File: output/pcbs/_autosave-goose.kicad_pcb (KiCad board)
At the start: 2 copper layers, 135.7 x 97.7 mm, 39 parts

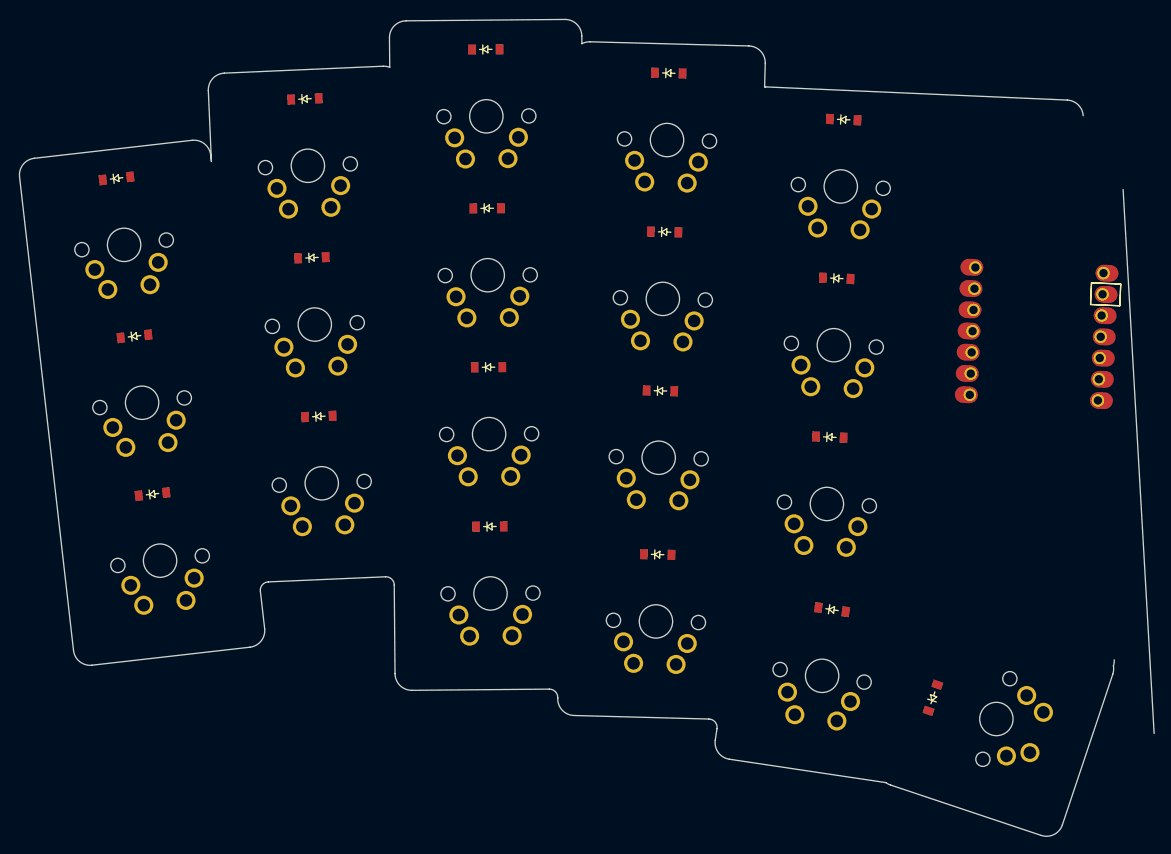
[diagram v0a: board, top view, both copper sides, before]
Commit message: partial
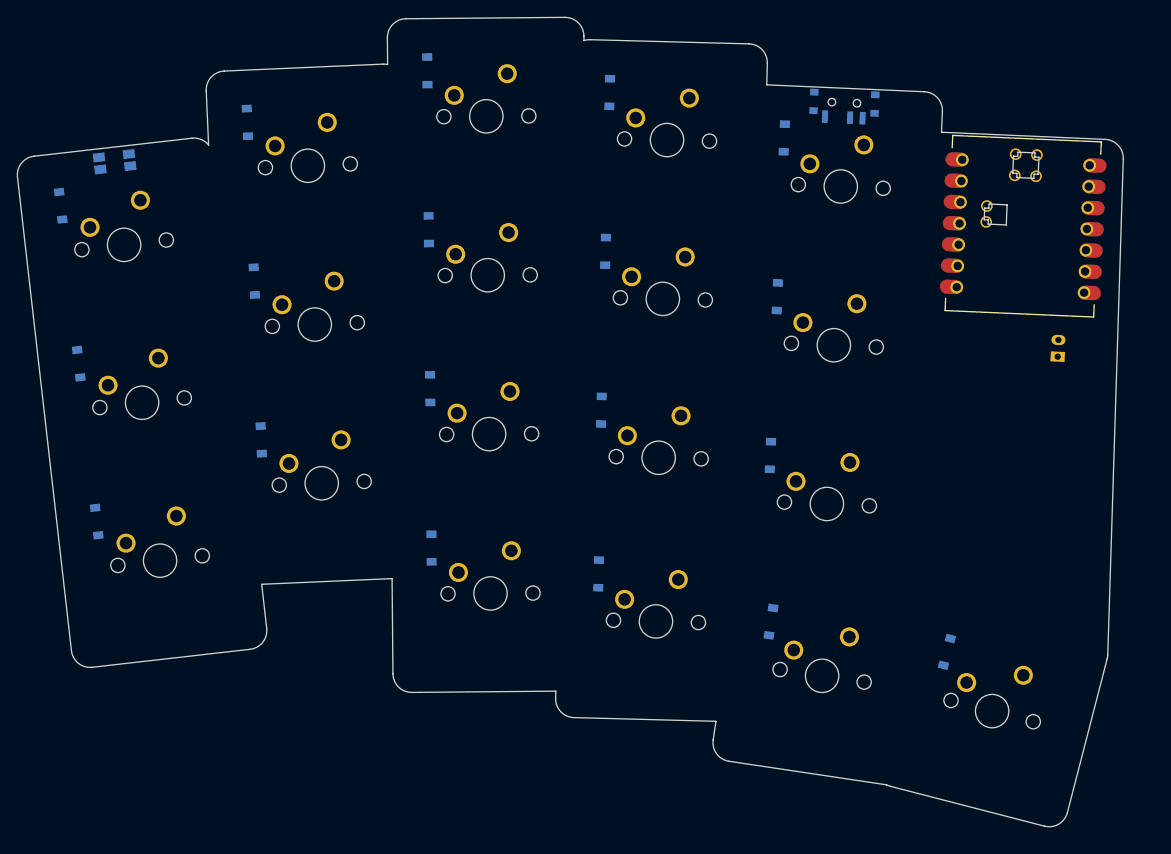
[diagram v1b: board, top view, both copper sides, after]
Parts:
- removed MCU1: , Seeeduino XIAO-MOUDLE14P-2.54-21X17.8MM tht maybe
- added ?: , power_switch, F.Cu at (261.7, 110.5)
- added BAT1 15 test: 18 line, BatteryPad, B.Cu at (287.2, 139.8)
- added SW1: , sw_reset_side, F.Cu at (174.4, 117.5)
- added _1: , Seeeduino XIAO nRF52840, F.Cu at (283.1, 125.2)
- moved D8 7.43 mm to (212.0, 125.6), turned to -89.5 degrees
- moved D10 7.43 mm to (232.6, 147.2), turned to -91.5 degrees
- moved D12 7.43 mm to (233.6, 109.2), turned to -91.5 degrees
- moved D11 7.43 mm to (233.1, 128.2), turned to -91.5 degrees
- moved D17 7.43 mm to (232.3, 166.8), turned to -91.5 degrees
- moved D1 7.43 mm to (172.3, 160.5), turned to -83.5 degrees
- moved D4 7.43 mm to (192.0, 150.8), turned to -87.5 degrees
- moved D9 7.43 mm to (211.8, 106.6), turned to -89.5 degrees
- moved D7 7.43 mm to (212.1, 144.6), turned to -89.5 degrees
- moved D13 7.43 mm to (252.8, 152.6), turned to -92.5 degrees
- moved D15 7.43 mm to (254.5, 114.7), turned to -92.5 degrees
- moved D14 7.43 mm to (253.7, 133.6), turned to -92.5 degrees
- moved D2 7.43 mm to (170.1, 141.7), turned to -83.5 degrees
- moved D3 7.43 mm to (168.0, 122.8), turned to -83.5 degrees
- moved D6 7.43 mm to (190.3, 112.8), turned to -87.5 degrees
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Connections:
- net index_bottom renamed C3_R2
- net index_home renamed C3_R1
- net index_top renamed C3_R0
- net inner_bottom renamed C4_R2
- net inner_home renamed C4_R1
- net inner_thumbs renamed C2_R3
- net inner_top renamed C4_R0
- net middle_bottom renamed C2_R2
- net middle_home renamed C2_R1
- net middle_thumbs renamed C1_R3
- net middle_top renamed C2_R0
- net outer_thumbs renamed C3_R3
- net pinkie_bottom renamed C0_R2
- net pinkie_home renamed C0_R1
- net pinkie_top renamed C0_R0
- net reach_thumbs renamed C4_R3
- net ring_bottom renamed C1_R2
- net ring_home renamed C1_R1
- net ring_top renamed C1_R0
- D1 pad 1: (no net) -> R2
- D10 pad 1: (no net) -> R2
- D11 pad 1: (no net) -> R1
- D12 pad 1: (no net) -> R0
- D13 pad 1: (no net) -> R2
- D14 pad 1: (no net) -> R1
- D15 pad 1: (no net) -> R0
- D16 pad 1: (no net) -> R3
- D17 pad 1: (no net) -> R3
- D18 pad 1: (no net) -> R3
- D19 pad 1: (no net) -> R3
- D2 pad 1: (no net) -> R1
- D3 pad 1: (no net) -> R0
- D4 pad 1: (no net) -> R2
- D5 pad 1: (no net) -> R1
- D6 pad 1: (no net) -> R0
- D7 pad 1: (no net) -> R2
- D8 pad 1: (no net) -> R1
- D9 pad 1: (no net) -> R0
- S1 pad 1: (no net) -> C0
- S10 pad 1: (no net) -> C3
- S11 pad 1: (no net) -> C3
- S12 pad 1: (no net) -> C3
- S13 pad 1: (no net) -> C4
- S14 pad 1: (no net) -> C4
- S15 pad 1: (no net) -> C4
- S16 pad 1: (no net) -> C1
- S17 pad 1: (no net) -> C2
- S18 pad 1: (no net) -> C3
- S19 pad 1: (no net) -> C4
- S2 pad 1: (no net) -> C0
- S3 pad 1: (no net) -> C0
- S4 pad 1: (no net) -> C1
- S5 pad 1: (no net) -> C1
- S6 pad 1: (no net) -> C1
- S7 pad 1: (no net) -> C2
- S8 pad 1: (no net) -> C2
- S9 pad 1: (no net) -> C2
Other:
- board size 135.7 x 97.7 mm -> 132.2 x 96.8 mm
